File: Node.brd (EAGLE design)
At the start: 38.1 x 38.1 mm, 70 parts, among them J1 AVR_SPI_PRG_6NS, J2 M04X2, Q1 PMR280UN, Q2 PMR280UN, Q3 PMR280UN, U1 ATMEGA32U4, U2 BLUETOOTH-RN41", U4 L3GD20, U9 RCLAMP0502A, X1 USBSMD

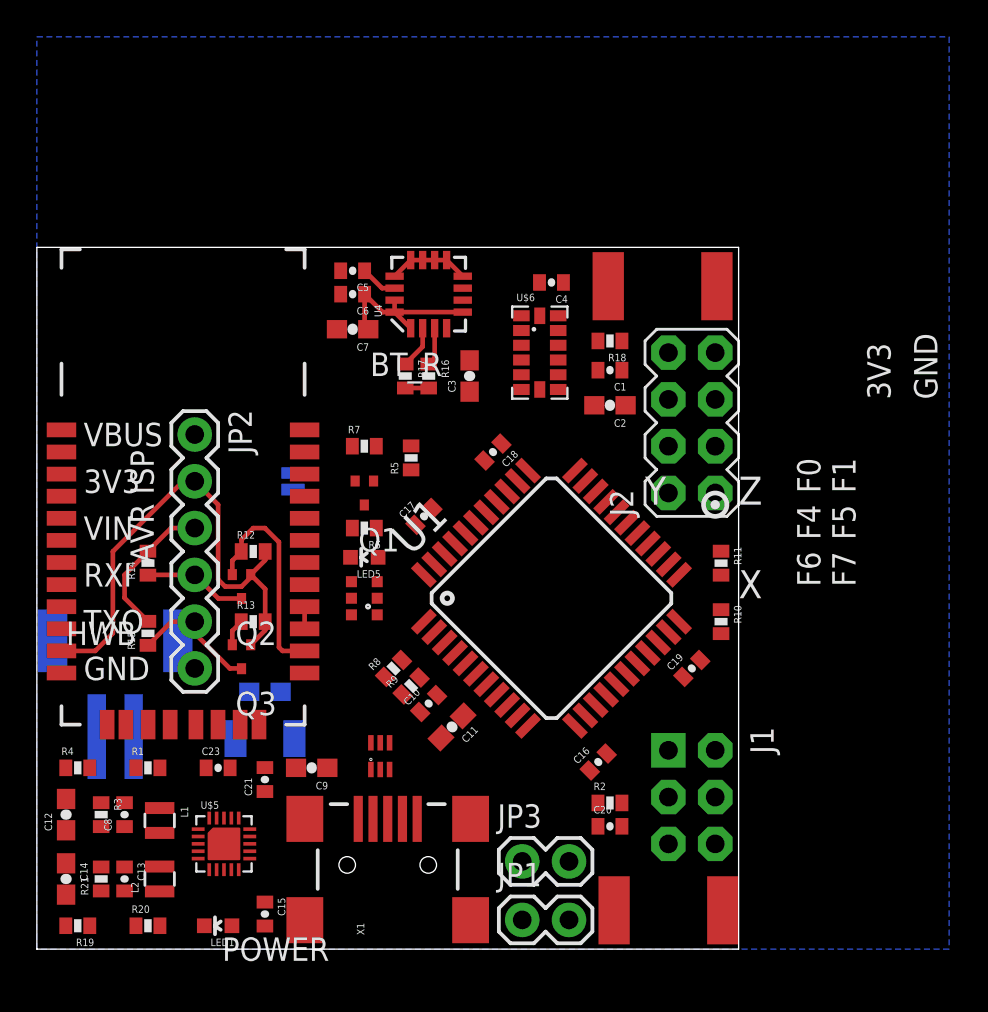
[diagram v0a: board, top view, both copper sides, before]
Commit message: mostly pass DRC
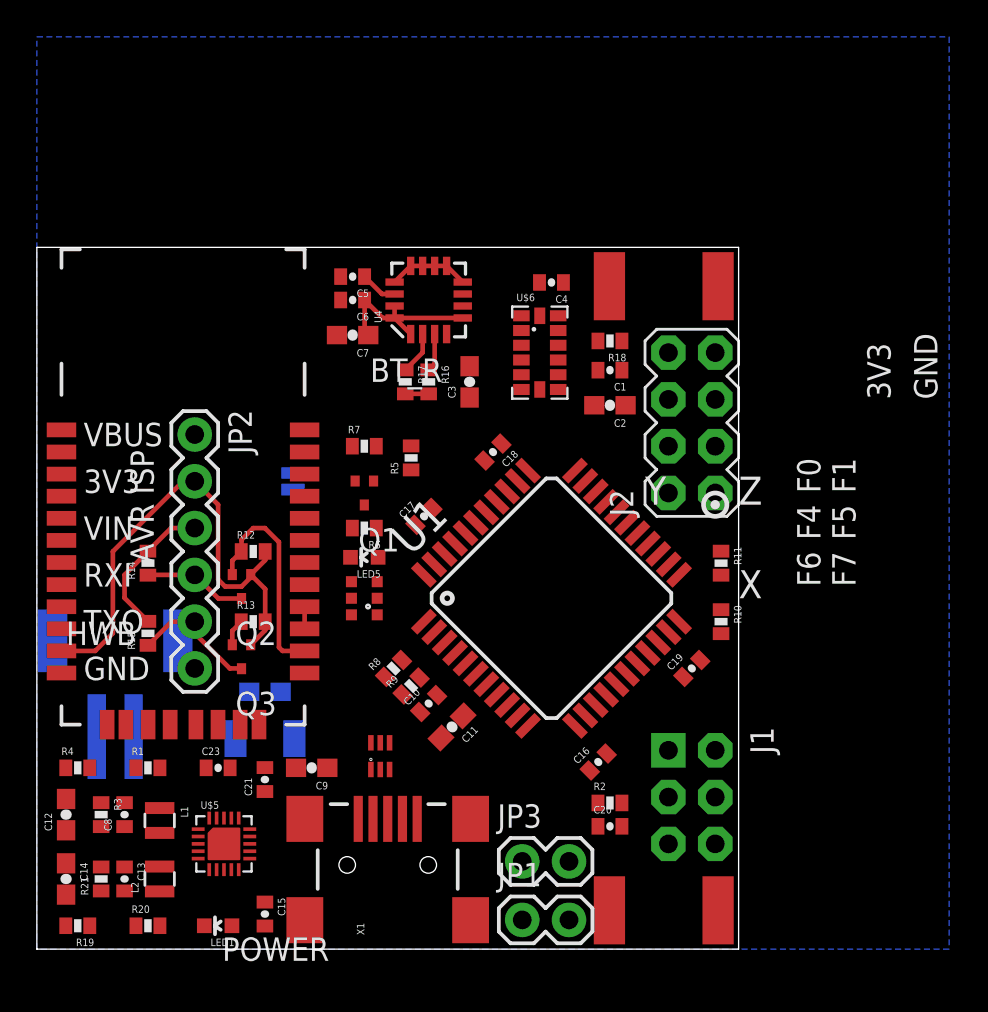
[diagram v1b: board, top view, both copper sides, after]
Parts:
- moved C6 0.32 mm to (17.1, 35.2)
- moved C7 0.32 mm to (17.1, 33.3)
- moved U4 0.32 mm to (21.3, 35.2)
- moved C3 0.32 mm to (23.5, 30.8)
- moved R16 0.32 mm to (21.3, 30.8)
- moved R17 0.32 mm to (20.0, 30.8)
- moved C5 0.32 mm to (17.1, 36.5)
- moved POWER 0.25 mm to (34.0, 2.11)
- moved HWB 0.06 mm to (34.0, 36.0)
